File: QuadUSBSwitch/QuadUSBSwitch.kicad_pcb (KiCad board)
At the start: 2 copper layers, 15 parts, among them J1 USB_A, J2 USB_A, J3 USB_OTG, J4 USB_OTG, J5 USB_OTG, J6 USB_OTG, J7 USB_OTG, SW1 SW_DIP_x04, U1 CH440G

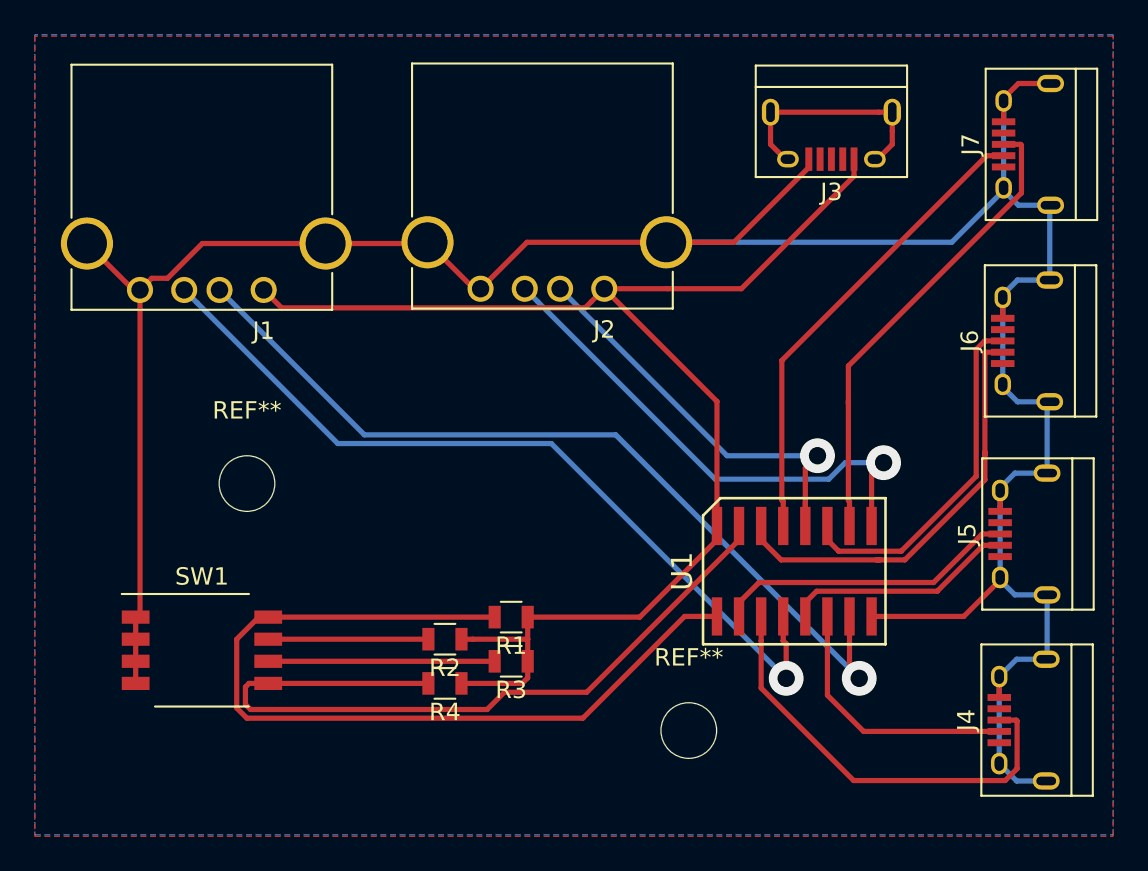
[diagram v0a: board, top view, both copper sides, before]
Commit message: update
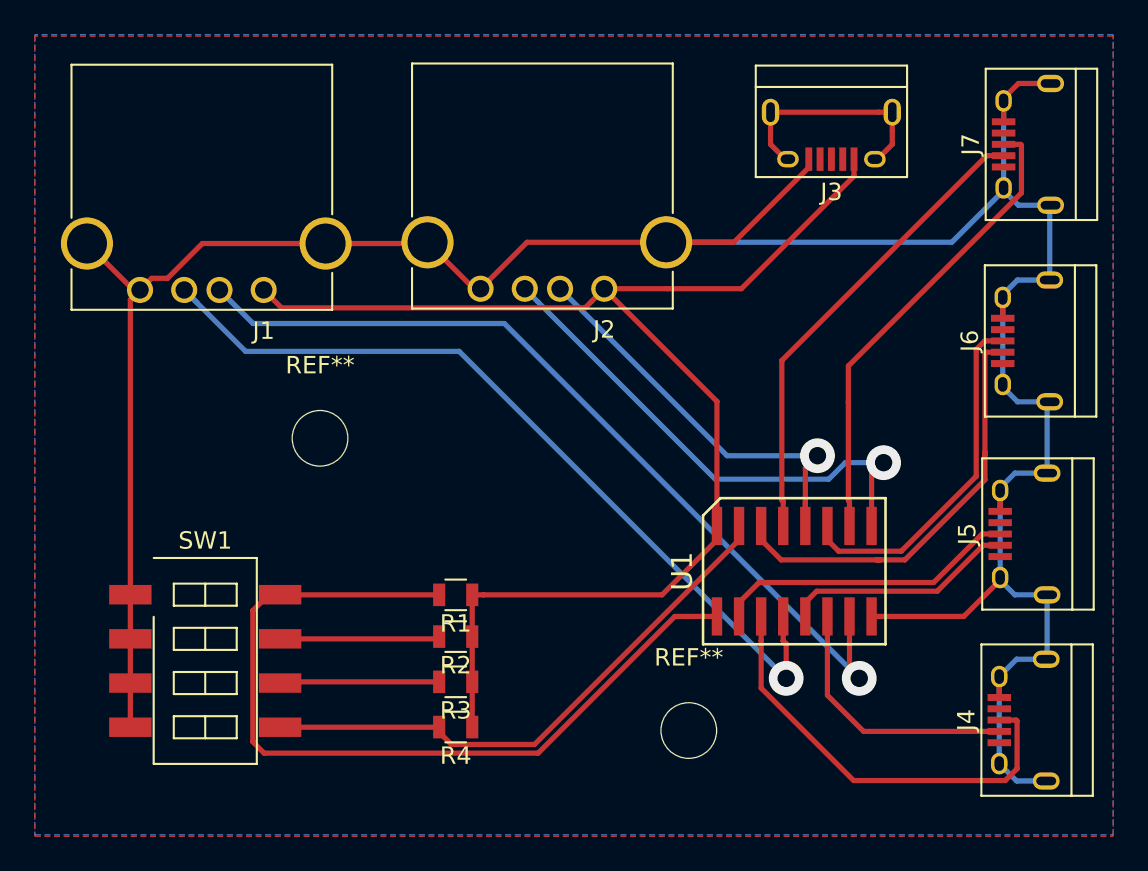
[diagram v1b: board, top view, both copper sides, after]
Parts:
- SW1: footprint Buttons_Switches_SMD:SW_DIP_x4_W7.62mm_Slide_Copal_CHS-B -> Buttons_Switches_SMD:SW_DIP_x4_W8.61mm_Slide_LowProfile
- moved REF** 4.94 mm to (86.4, 81.2)
- moved R1 3.44 mm to (94.2, 90.2)
- moved R3 3.40 mm to (94.2, 95.2)
- moved R4 2.59 mm to (94.2, 97.8)
- moved SW1 0.64 mm to (79.8, 94.0)
- moved R2 0.64 mm to (94.2, 92.6)
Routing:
- net Net-(R4-Pad2): track 45.4 -> 32.7 mm
- net Net-(R3-Pad2): track 13.0 -> 9.17 mm
- net GND: track 162.7 -> 165.4 mm
- net VBUS: track 79.9 -> 78.6 mm
- net Net-(J1-Pad3): track 47.5 -> 48.6 mm
- net Net-(R1-Pad2): track 49.6 -> 48.9 mm
